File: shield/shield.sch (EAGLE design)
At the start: 24 parts, among them IC1 MCP2515-E/SO, IC2 MCP2562, IC3 LM2595NDH, IC4 PESD1CAN

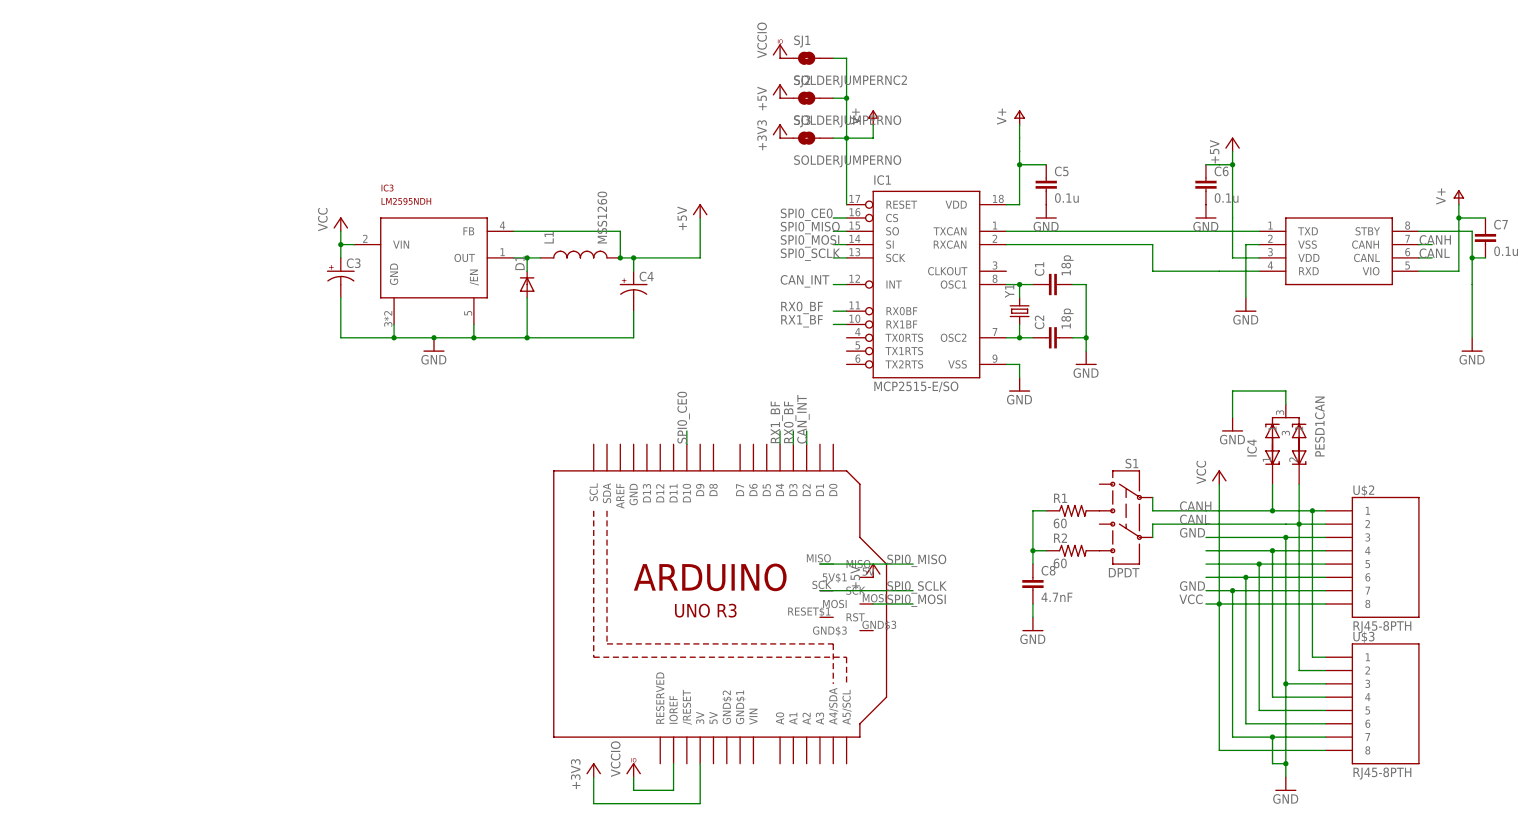
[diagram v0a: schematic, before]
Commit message: Minor changes to shield, rpi board, and cape
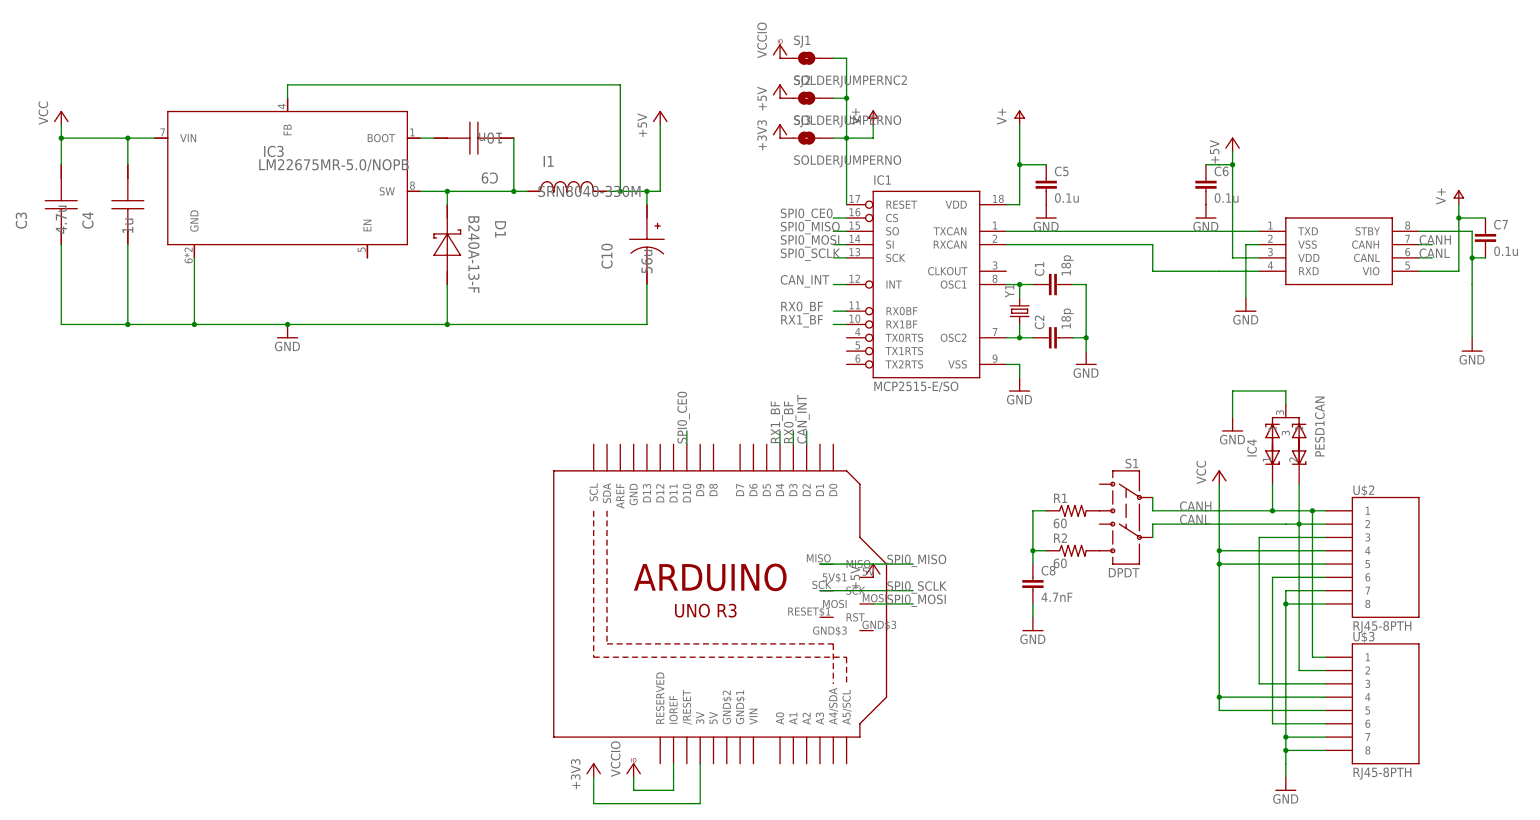
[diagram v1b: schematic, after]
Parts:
- removed L1: MSS1260, nickparts:MSS1260
- added C10: 56u, nickparts:10SVP56M
- added C9: 10n, nickparts:C0805C103K5RACTU
- added I1: SRN8040-330M, nickparts:SRN8040-330M
- C3: value (none) -> 4.7u; device SparkFun-Capacitors:CAP_POLG -> nickparts:GRM31CR71H475KA12L
- C4: value (none) -> 1u; device SparkFun-Capacitors:CAP_POLE -> nickparts:GMK212B7105KG-T
- D1: value (none) -> B240A-13-F; device SparkFun-DiscreteSemi:DIODESMA-ALT -> nickparts:B240A-13-F
- IC3: value LM2595NDH -> LM22675MR-5.0/NOPB; device nickparts:LM2595NDH -> nickparts:LM22675MR-5.0/NOPB
- U$1: value ARDUINO_R3_ICSP -> ARDUINO_R3_ICSPNODIM; device adafruit:ARDUINO_R3_ICSP -> nickparts:ARDUINO_R3_ICSPNODIM
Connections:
- net N$1 renamed RXCAN
- removed net N$11: U$2.5, U$3.5
- removed net N$6: D1.C, IC3.OUT, L1.1
- new net N$9: U$2.3, U$3.3
- new net SWOUT: C9.2, D1.K, I1.2, IC3.SW
- net +5V: now also C10.+, I1.1; no longer C4.+, L1.2
- net GND: now also C10.-, C3.2, C4.2, U$2.8, U$3.8; no longer C3.-, C4.-, IC3./EN, U$2.3, U$3.3
- net N$10: now also C9.1, IC3.BOOT; no longer U$2.4, U$3.4
- net VCC: now also C3.1, C4.1, U$2.4, U$2.5, U$3.4, U$3.5; no longer C3.+, U$2.8, U$3.8
